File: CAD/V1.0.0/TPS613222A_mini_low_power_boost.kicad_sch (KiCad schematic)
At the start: 17 parts, among them K1 HEADER_MALE_1X1, K2 TERMINAL_KF235-5.0-2P, K3 HEADER_MALE_1X1, K4 HEADER_MALE_1X1, K5 TERMINAL_KF235-5.0-2P, K6 HEADER_MALE_1X1, U1 TPS613222A

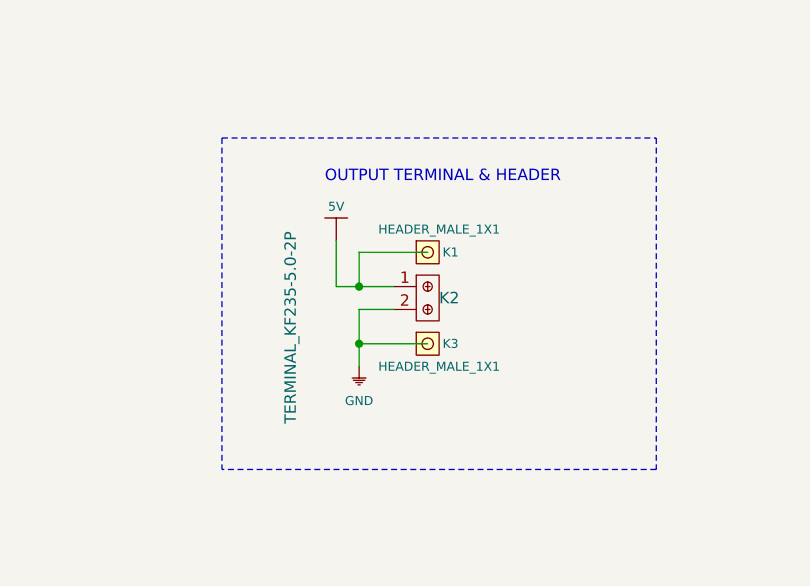
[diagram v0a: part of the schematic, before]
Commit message: Updating open source files.
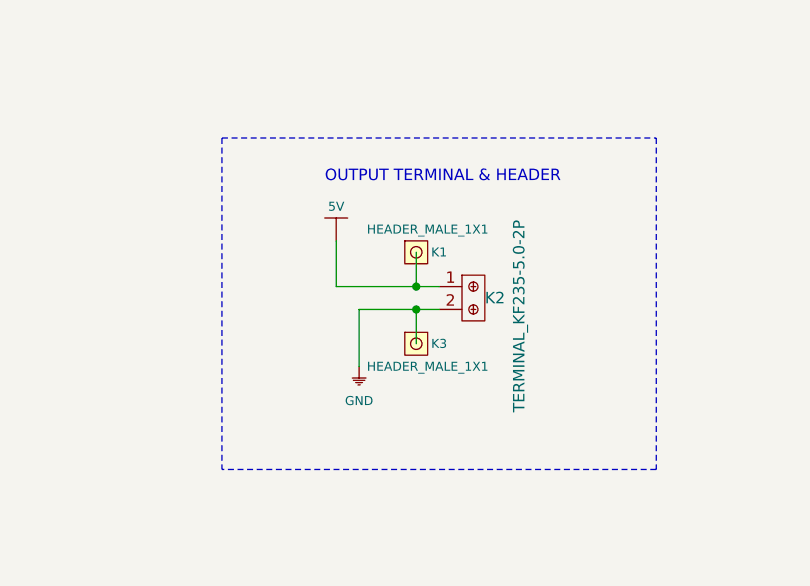
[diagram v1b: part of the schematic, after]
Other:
- moved on the sheet: K1, K2, K3
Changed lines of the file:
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@@
   (junction (at 67.945 67.056) (diameter 0.9144) (color 0 0 0 0))
   (junction (at 81.915 55.88) (diameter 0.9144) (color 0 0 0 0))
-  (junction (at 86.36 119.38) (diameter 0.9144) (color 0 0 0 0))
-  (junction (at 86.36 125.73) (diameter 0.9144) (color 0 0 0 0))
+  (junction (at 92.71 119.38) (diameter 0.9144) (color 0 0 0 0))
+  (junction (at 92.71 121.92) (diameter 0.9144) (color 0 0 0 0))
   (junction (at 137.795 59.69) (diameter 0.9144) (color 0 0 0 0))
   (junction (at 204.47 54.61) (diameter 0.9144) (color 0 0 0 0))
@@
     (stroke (width 0) (type solid) (color 0 0 0 0))
   )
-  (wire (pts (xy 83.82 119.38) (xy 86.36 119.38))
-    (stroke (width 0) (type solid) (color 0 0 0 0))
-  )
-  (wire (pts (xy 86.36 115.57) (xy 86.36 119.38))
-    (stroke (width 0) (type solid) (color 0 0 0 0))
-  )
-  (wire (pts (xy 86.36 119.38) (xy 90.17 119.38))
-    (stroke (width 0) (type solid) (color 0 0 0 0))
-  )
-  (wire (pts (xy 86.36 121.92) (xy 86.36 125.73))
-    (stroke (width 0) (type solid) (color 0 0 0 0))
-  )
-  (wire (pts (xy 86.36 125.73) (xy 86.36 128.27))
+  (wire (pts (xy 83.82 119.38) (xy 92.71 119.38))
+    (stroke (width 0) (type solid) (color 0 0 0 0))
+  )
+  (wire (pts (xy 86.36 121.92) (xy 86.36 128.27))
+    (stroke (width 0) (type solid) (color 0 0 0 0))
+  )
+  (wire (pts (xy 86.36 121.92) (xy 92.71 121.92))
     (stroke (width 0) (type solid) (color 0 0 0 0))
   )
@@
     (stroke (width 0) (type solid) (color 0 0 0 0))
   )
-  (wire (pts (xy 90.17 121.92) (xy 86.36 121.92))
-    (stroke (width 0) (type solid) (color 0 0 0 0))
-  )
-  (wire (pts (xy 93.98 115.57) (xy 86.36 115.57))
-    (stroke (width 0) (type solid) (color 0 0 0 0))
-  )
-  (wire (pts (xy 93.98 125.73) (xy 86.36 125.73))
+  (wire (pts (xy 92.71 115.57) (xy 92.71 119.38))
+    (stroke (width 0) (type solid) (color 0 0 0 0))
+  )
+  (wire (pts (xy 92.71 119.38) (xy 95.25 119.38))
+    (stroke (width 0) (type solid) (color 0 0 0 0))
+  )
+  (wire (pts (xy 92.71 121.92) (xy 92.71 125.73))
+    (stroke (width 0) (type solid) (color 0 0 0 0))
+  )
+  (wire (pts (xy 92.71 121.92) (xy 95.25 121.92))
     (stroke (width 0) (type solid) (color 0 0 0 0))
   )
@@
     (pin "1")
   )
-  (symbol (lib_id "e-radionica.com schematics:HEADER_MALE_1X1") (at 93.98 115.57 0) (unit 1)
-    (in_bom yes) (on_board yes)
-    (property "Reference" "K1" (id 0) (at 96.52 115.57 0)
-      (effects (font (size 1 1)))
-    )
-    (property "Value" "HEADER_MALE_1X1" (id 1) (at 95.25 113.03 0)
-      (effects (font (size 1 1)))
-    )
-    (property "Footprint" "e-radionica.com footprinti:HEADER_MALE_1X1" (id 2) (at 93.98 115.57 0)
-      (effects (font (size 1 1)) hide)
-    )
-    (property "Datasheet" "" (id 3) (at 93.98 115.57 0)
-      (effects (font (size 1 1)) hide)
-    )
-    (pin "1")
-  )
-  (symbol (lib_id "e-radionica.com schematics:HEADER_MALE_1X1") (at 93.98 125.73 0) (unit 1)
-    (in_bom yes) (on_board yes)
-    (property "Reference" "K3" (id 0) (at 96.52 125.73 0)
-      (effects (font (size 1 1)))
-    )
-    (property "Value" "HEADER_MALE_1X1" (id 1) (at 95.25 128.27 0)
-      (effects (font (size 1 1)))
-    )
-    (property "Footprint" "e-radionica.com footprinti:HEADER_MALE_1X1" (id 2) (at 93.98 125.73 0)
-      (effects (font (size 1 1)) hide)
-    )
-    (property "Datasheet" "" (id 3) (at 93.98 125.73 0)
+  (symbol (lib_id "e-radionica.com schematics:HEADER_MALE_1X1") (at 92.71 115.57 0) (unit 1)
+    (in_bom yes) (on_board yes)
+    (property "Reference" "K1" (id 0) (at 95.25 115.57 0)
+      (effects (font (size 1 1)))
+    )
+    (property "Value" "HEADER_MALE_1X1" (id 1) (at 93.98 113.03 0)
+      (effects (font (size 1 1)))
+    )
+    (property "Footprint" "e-radionica.com footprinti:HEADER_MALE_1X1" (id 2) (at 92.71 115.57 0)
+      (effects (font (size 1 1)) hide)
+    )
+    (property "Datasheet" "" (id 3) (at 92.71 115.57 0)
+      (effects (font (size 1 1)) hide)
+    )
+    (pin "1")
+  )
+  (symbol (lib_id "e-radionica.com schematics:HEADER_MALE_1X1") (at 92.71 125.73 0) (unit 1)
+    (in_bom yes) (on_board yes)
+    (property "Reference" "K3" (id 0) (at 95.25 125.73 0)
+      (effects (font (size 1 1)))
+    )
+    (property "Value" "HEADER_MALE_1X1" (id 1) (at 93.98 128.27 0)
+      (effects (font (size 1 1)))
+    )
+    (property "Footprint" "e-radionica.com footprinti:HEADER_MALE_1X1" (id 2) (at 92.71 125.73 0)
+      (effects (font (size 1 1)) hide)
+    )
+    (property "Datasheet" "" (id 3) (at 92.71 125.73 0)
       (effects (font (size 1 1)) hide)
     )
@@
     (pin "2")
   )
-  (symbol (lib_id "e-radionica.com schematics:TERMINAL_KF235-5.0-2P") (at 93.98 120.65 0) (unit 1)
-    (in_bom yes) (on_board yes)
-    (property "Reference" "K2" (id 0) (at 95.25 120.6499 0)
+  (symbol (lib_id "e-radionica.com schematics:TERMINAL_KF235-5.0-2P") (at 99.06 120.65 0) (unit 1)
+    (in_bom yes) (on_board yes)
+    (property "Reference" "K2" (id 0) (at 100.33 120.6499 0)
       (effects (font (size 1.27 1.27)) (justify left))
     )
-    (property "Value" "TERMINAL_KF235-5.0-2P" (id 1) (at 78.74 134.6199 90)
+    (property "Value" "TERMINAL_KF235-5.0-2P" (id 1) (at 104.14 133.3499 90)
       (effects (font (size 1.27 1.27)) (justify left))
     )
-    (property "Footprint" "e-radionica.com footprinti:TERMINAL_KF235-5.0-2P" (id 2) (at 93.98 120.65 0)
-      (effects (font (size 1.27 1.27)) hide)
-    )
-    (property "Datasheet" "" (id 3) (at 93.98 120.65 0)
-      (effects (font (size 1.27 1.27)) hide)
-    )
+    (property "Footprint" "e-radionica.com footprinti:TERMINAL_KF235-5.0-2P" (id 2) (at 99.06 120.65 0)
+      (effects (font (size 1.27 1.27)) hide)
+    )
+    (property "Datasheet" "" (id 3) (at 99.06 120.65 0)
+      (effects (font (size 1.27 1.27)) hide)
+    )
